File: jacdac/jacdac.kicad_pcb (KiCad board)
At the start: 2 copper layers, 62.9 x 33.4 mm, 15 parts, among them J1 Conn_02x03_Odd_Even, J2 Conn_02x03_Odd_Even, J3 Audio_Jack_TRRS, J4 Audio_Jack_TRRS, J5 Audio_Jack_TRRS, J6 Audio_Jack_TRRS

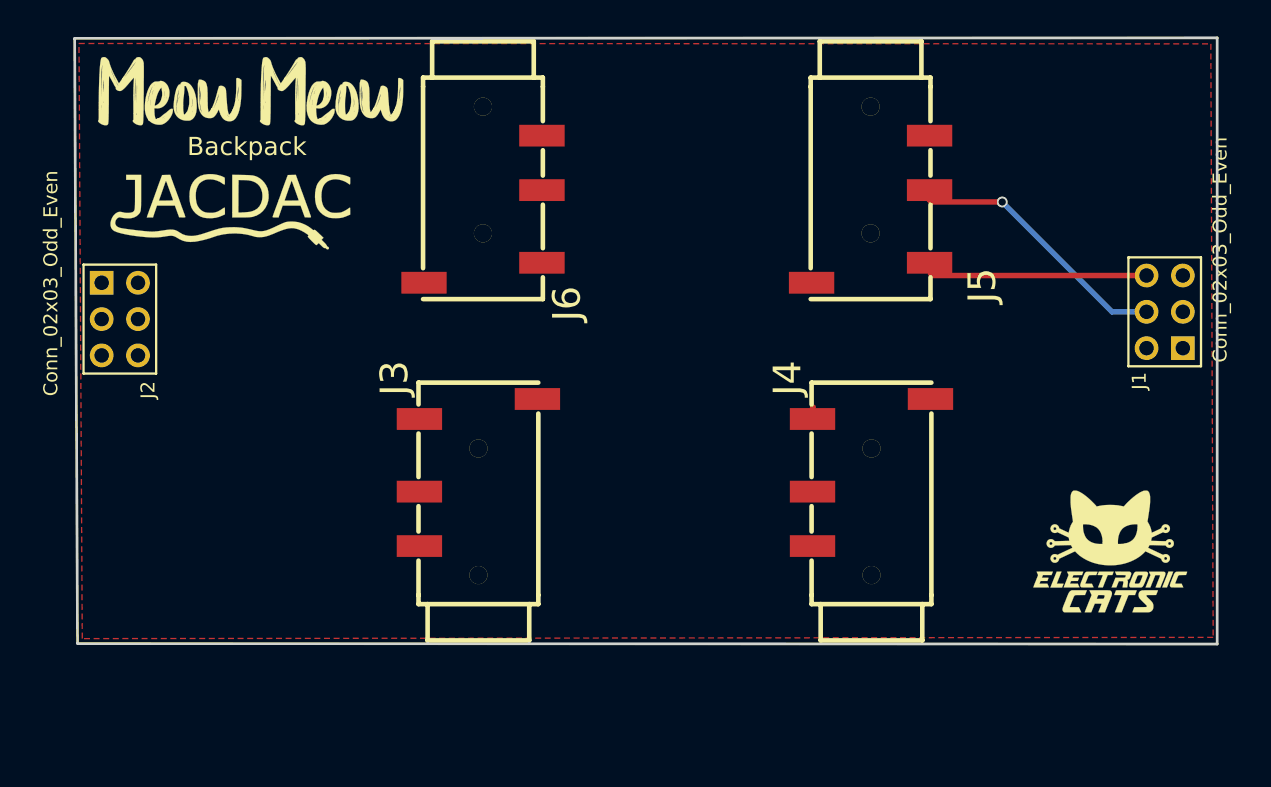
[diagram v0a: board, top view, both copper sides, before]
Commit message: update pcb
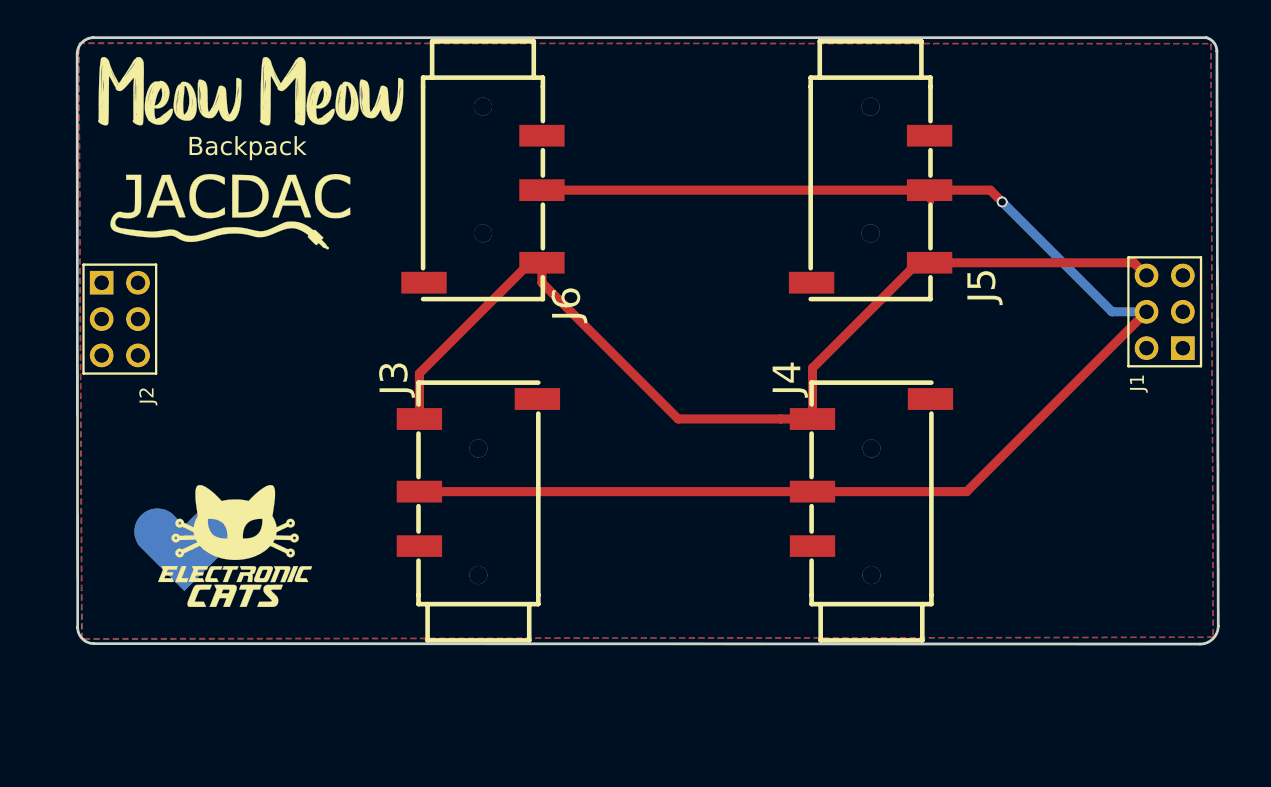
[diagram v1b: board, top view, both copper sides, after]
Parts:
- added G***: LOGO, Aesthetics:jacdac_logo_14x6, B.Cu at (129.0, 47.8)
- added svg2mod: G***, svg2mod, B.Cu at (83.7, 64.1)
- moved G*** 48.2 mm to (86.5, 63.9)
- moved G*** 8.49 mm to (94.3, 64.7)
- moved REF*** 4.25 mm to (105.0, 64.6)
- moved REF*** 4.05 mm to (114.2, 64.0)
- moved REF*** 1.41 mm to (127.8, 63.7)
- moved REF*** 1.04 mm to (136.0, 63.7)
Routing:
- net /JACDAC_TX: track 15.1 -> 81.0 mm
- net VCC: track 12.0 -> 55.7 mm
- added copper zone on B.Cu, net GND
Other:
- board size 62.9 x 33.4 mm -> 62.8 x 33.4 mm
- net class source added: clearance 0.2, trace_width 0.5, via_dia 0.6, via_drill 0.4
- board text added: "- Connect with audio cable 3.5mm"
- board text added: "Made with in México"
- board text removed: "Backpack JACDAC"
- board text removed: "JACDAC - Connect with audio cable 3.5mm"

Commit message: update pcb
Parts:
- J1: value Conn_02x03_Odd_Even -> Conn1
- J2: value Conn_02x03_Odd_Even -> Conn2
- moved G*** 2.94 mm to (121.4, 39.4)
- moved G*** 1.73 mm to (129.8, 46.2)
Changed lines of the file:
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@@
   )
   (module LOGO (layer B.Cu)
-    (at 124.35 39.6 180)
+    (at 121.425 39.35 180)
     (fp_text reference G*** (at 0 0 180) (layer B.SilkS) hide
       (effects (font (size 1.524 1.524) (thickness 0.3)) (justify mirror))
@@
       (effects (font (size 0.77216 0.77216) (thickness 0.065024)) (justify left bottom))
     )
-    (fp_text value Conn_02x03_Odd_Even (at 3.55 1.35) (layer B.SilkS)
+    (fp_text value Conn1 (at -4.225 1.9) (layer B.SilkS)
       (effects (font (size 0.77216 0.77216) (thickness 0.065024)) (justify left bottom mirror))
     )
@@
       (effects (font (size 0.77216 0.77216) (thickness 0.065024)) (justify left bottom))
     )
-    (fp_text value Conn_02x03_Odd_Even (at -3.275 -1.65 180) (layer B.SilkS)
+    (fp_text value Conn2 (at 4.15 -1.925 180) (layer B.SilkS)
       (effects (font (size 0.77216 0.77216) (thickness 0.065024)) (justify left bottom mirror))
     )
@@
   )
   (module Aesthetics:jacdac_logo_14x6 (layer B.Cu)
-    (at 129.025 47.8 180)
+    (at 129.75 46.225 180)
     (fp_text reference G*** (at 0 0 180) (layer B.SilkS) hide
       (effects (font (size 1.524 1.524) (thickness 0.3)) (justify mirror))
@@
     (effects (font (size 1 1) (thickness 0.25)) (justify mirror))
   )
-  (gr_text "Backpack " (at 129.7 44.55) (layer B.SilkS)
+  (gr_text "Backpack " (at 130.525 43.575) (layer B.SilkS)
     (effects (font (size 1.3 1.3) (thickness 0.3) italic) (justify mirror))
   )

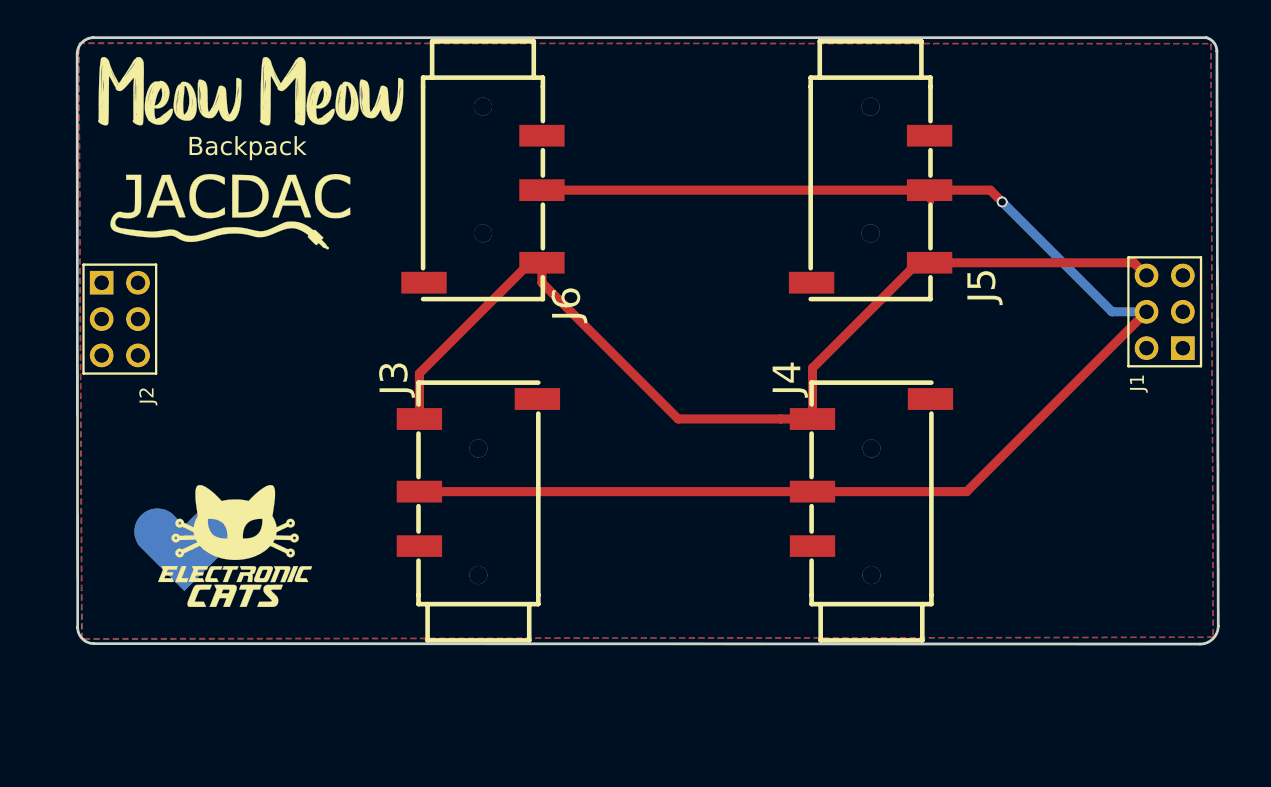
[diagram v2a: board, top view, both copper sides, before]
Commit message: mode star
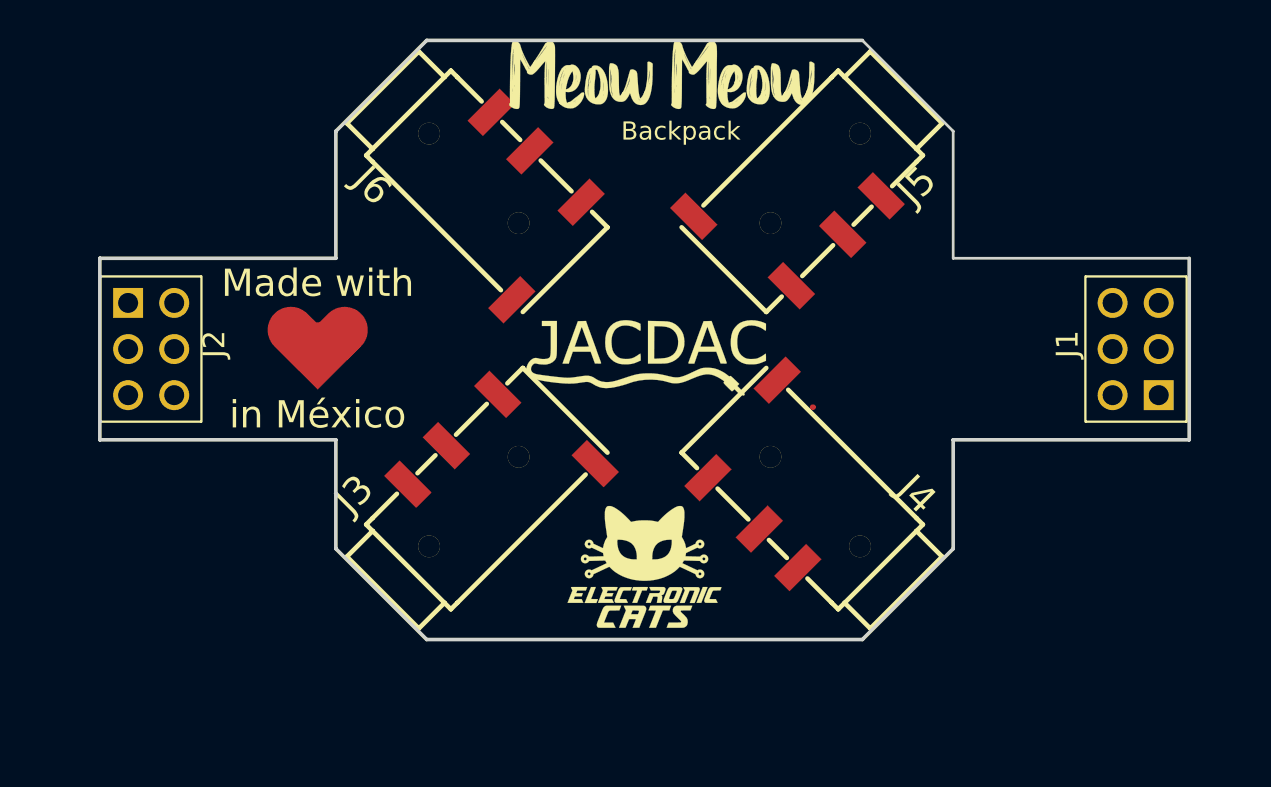
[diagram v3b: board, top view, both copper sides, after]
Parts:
- removed the G*** at (86.5, 63.9)
- removed the G*** at (94.3, 64.7)
- removed the REF*** at (127.8, 63.7)
- added G***: LOGO, Aesthetics:electronic_cats_logo_8x6, F.Cu at (109.0, 65.0)
- J1, J2: footprint Pines:62000621121 -> Pines:61300621121
- svg2mod: moved to F.Cu
- moved REF*** 35.1 mm to (101.0, 65.0)
- moved G*** 24.3 mm to (109.0, 53.0)
- moved G*** 22.7 mm to (110.0, 38.0)
- moved G*** 21.0 mm to (110.0, 39.0)
- moved G*** 16.0 mm to (108.0, 48.0)
- moved svg2mod 13.3 mm to (91.0, 53.0), turned to 0 degrees
- moved J6 4.54 mm to (96.0, 40.0), turned to 315 degrees
- moved J3 4.36 mm to (96.0, 65.0), turned to 45 degrees
- moved REF*** 3.05 mm to (108.0, 65.0)
- moved J1 2.60 mm to (136.1, 53.0)
- moved J2 2.39 mm to (81.8, 53.0)
- moved J4 2.11 mm to (122.0, 65.0), turned to 135 degrees
- moved REF*** 2.03 mm to (116.0, 65.0)
- moved J5 2.03 mm to (122.0, 40.0), turned to 225 degrees
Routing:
- net /JACDAC_TX: track 81.0 -> 0.00 mm, vias 1 -> 0
- net VCC: track 55.7 -> 0.00 mm
- removed copper zone on B.Cu, net GND
- removed copper zone on F.Cu, net GND
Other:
- board size 62.8 x 33.4 mm -> 60 x 33 mm

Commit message: version for test
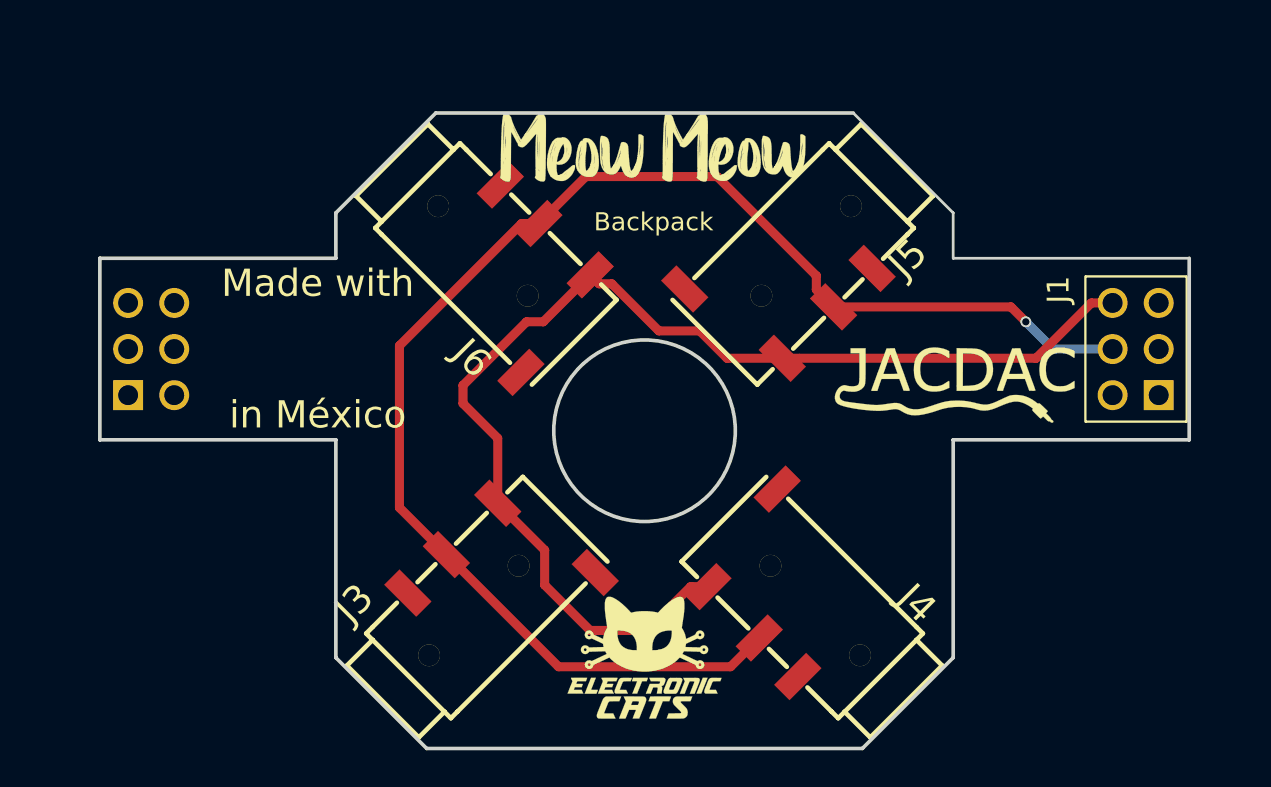
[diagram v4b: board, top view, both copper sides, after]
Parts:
- removed the G*** at (108.0, 48.0)
- removed the svg2mod at (91.0, 53.0)
- added G***: LOGO, Aesthetics:meowmeow_logo_21x8, B.Cu at (108.0, 48.0)
- added svg2mod: G***, Aesthetics:heart_trans, F.Cu at (91.0, 53.0)
- J2: moved to B.Cu
- moved G*** 17.1 mm to (126.0, 54.5)
- moved REF*** 7.02 mm to (115.5, 72.0)
- moved REF*** 7.00 mm to (108.0, 72.0)
- moved REF*** 6.50 mm to (101.0, 71.5)
- moved J3 6.00 mm to (96.0, 71.0)
- moved J4 6.00 mm to (122.0, 71.0)
- moved G*** 5.00 mm to (109.0, 70.0)
- moved G*** 4.03 mm to (109.5, 42.0)
- moved J5 4.03 mm to (121.5, 44.0)
- moved J6 4.03 mm to (96.5, 44.0)
- moved G*** 3.00 mm to (110.0, 42.0)
- turned J2 to 90 degrees
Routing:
- net /JACDAC_TX: track 0.00 -> 80.5 mm, vias 0 -> 1
- net VCC: track 0.00 -> 65.4 mm
- added copper zone on B.Cu, net GND
- added copper zone on F.Cu, net GND
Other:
- board size 60 x 33 mm -> 60 x 35 mm
- board text added: "Connect with audio cable 3.5mm"
- board text removed: "- Connect with audio cable 3.5mm"
